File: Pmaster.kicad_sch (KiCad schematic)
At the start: 158 parts, among them U1 Pico, U2 Pico, U3 Pico, U4 Pico, U5 LM4040LP-3

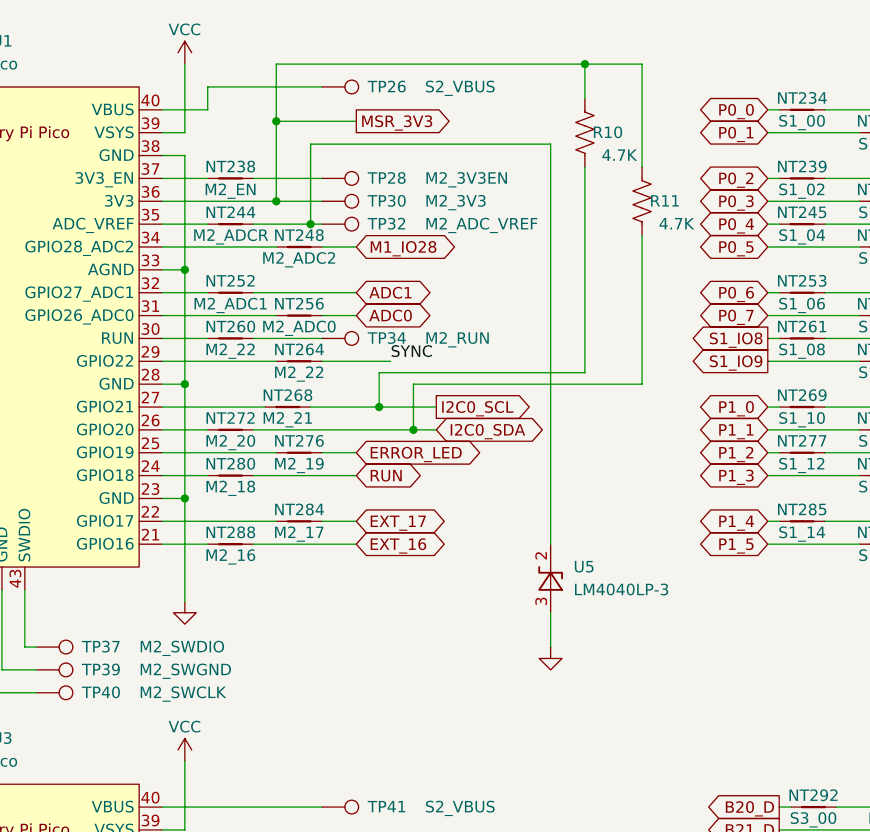
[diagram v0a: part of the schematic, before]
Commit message: update
Correction of small error
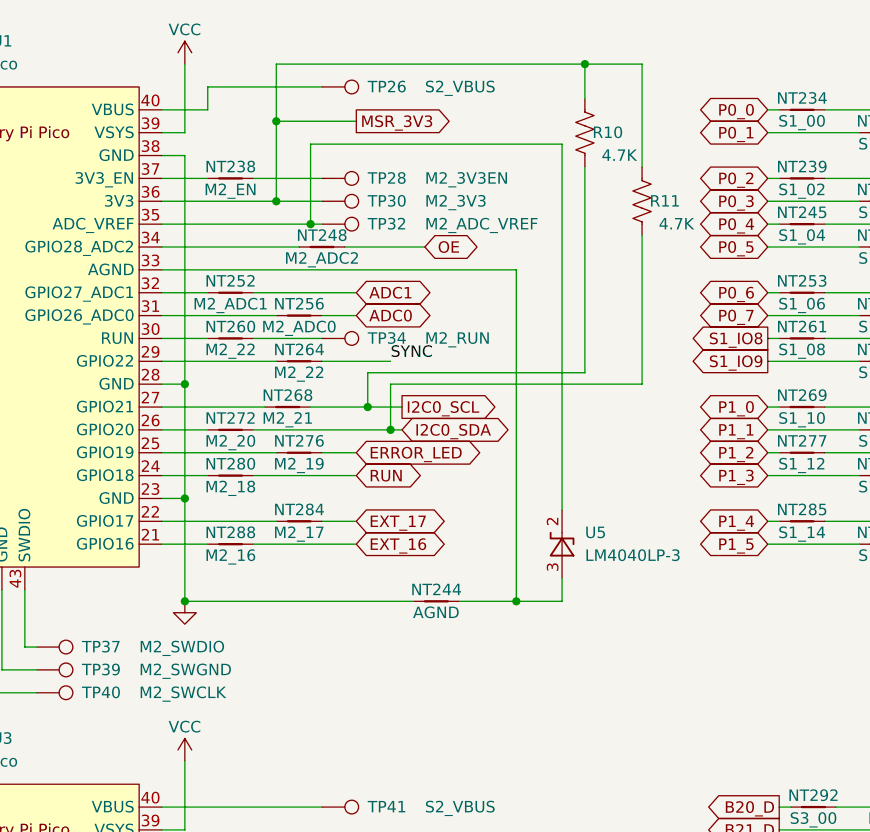
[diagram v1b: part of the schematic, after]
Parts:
- NT244: value M2_ADCR -> AGND
- R1, R10, R11, R12, R13, R14, R16, R17: footprint Resistor_THT:R_Axial_DIN0309_L9.0mm_D3.2mm_P12.70mm_Horizontal -> Resistor_THT:R_Axial_DIN0207_L6.3mm_D2.5mm_P10.16mm_Horizontal
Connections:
- net GND: now also NT244.2; no longer U1.33 (AGND), U5.3 (A)
- net at TP32.1, U5.2 (K): now also U1.35 (ADC_VREF); no longer NT244.2
- net at NT244.1: now also U1.33 (AGND), U5.3 (A); no longer U1.35 (ADC_VREF)
- net M1_IO28 renamed OE
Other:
- moved on the sheet: NT248, U5
